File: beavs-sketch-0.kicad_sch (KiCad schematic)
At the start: 31 parts, among them J1 USB_C_Receptacle_USB2.0_16P, J3 Conn_01x02, J5 Conn_01x02, Q1 SiS402DN, Q2 SiS402DN, U15 SN74LVC8T245, U16 SRV05-4, U17 SRV05-4, U19 LM74502, U7 AMS1117-3.3, U8 AMS1117-5.0

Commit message: I may be stupid
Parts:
- removed C46: 220n, Capacitor_SMD:C_0402_1005Metric, symbol Device:C_Small
- removed R2: 100, Resistor_SMD:R_0402_1005Metric, symbol Device:R_Small
- removed U19: LM74502, Package_TO_SOT_SMD:SOT-23-8, symbol beavs-symbols:LM74502
- added Q3: AO3401A, Package_TO_SOT_SMD:SOT-23, symbol Transistor_FET:AO3401A
- added R14: R_Small, Resistor_SMD:R_0402_1005Metric, symbol Device:R_Small
- added R2: R, Resistor_SMD:R_0805_2012Metric, symbol Device:R
- added U19: LM74700, Package_TO_SOT_SMD:SOT-23-6, symbol Power_Management:LM74700
- C45: value 220n -> C_Small; LCSC C16772 -> (none)
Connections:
- net +BATT: now also U19.4 (CATHODE)
- net GND: now also U19.2 (GND)
- net at J3.2 (Pin_2), Q1.5 (D): now also R2.1
- net at Q1.4 (G): now also Q3.3 (D), R14.2; no longer Q2.4 (G)
- net at C45.1: now also Q1.1 (S), Q1.2 (S), Q1.3 (S), Q2.1 (S), Q2.2 (S), Q2.3 (S), R14.1, R2.2, U19.6 (ANODE)
- net at C45.2: now also U19.1 (VCAP)
- new net: Q2.4 (G), Q3.2 (S), U19.5 (GATE)
- new net mcu/SERVO_POWER_EN: Q3.1 (G)
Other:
- sheet mcu ports: added SERVO_POWER_EN; removed none
- moved on the sheet: C15, C16, C17, C18, D1, D2, D3, D4, D5, D6, D7, D8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

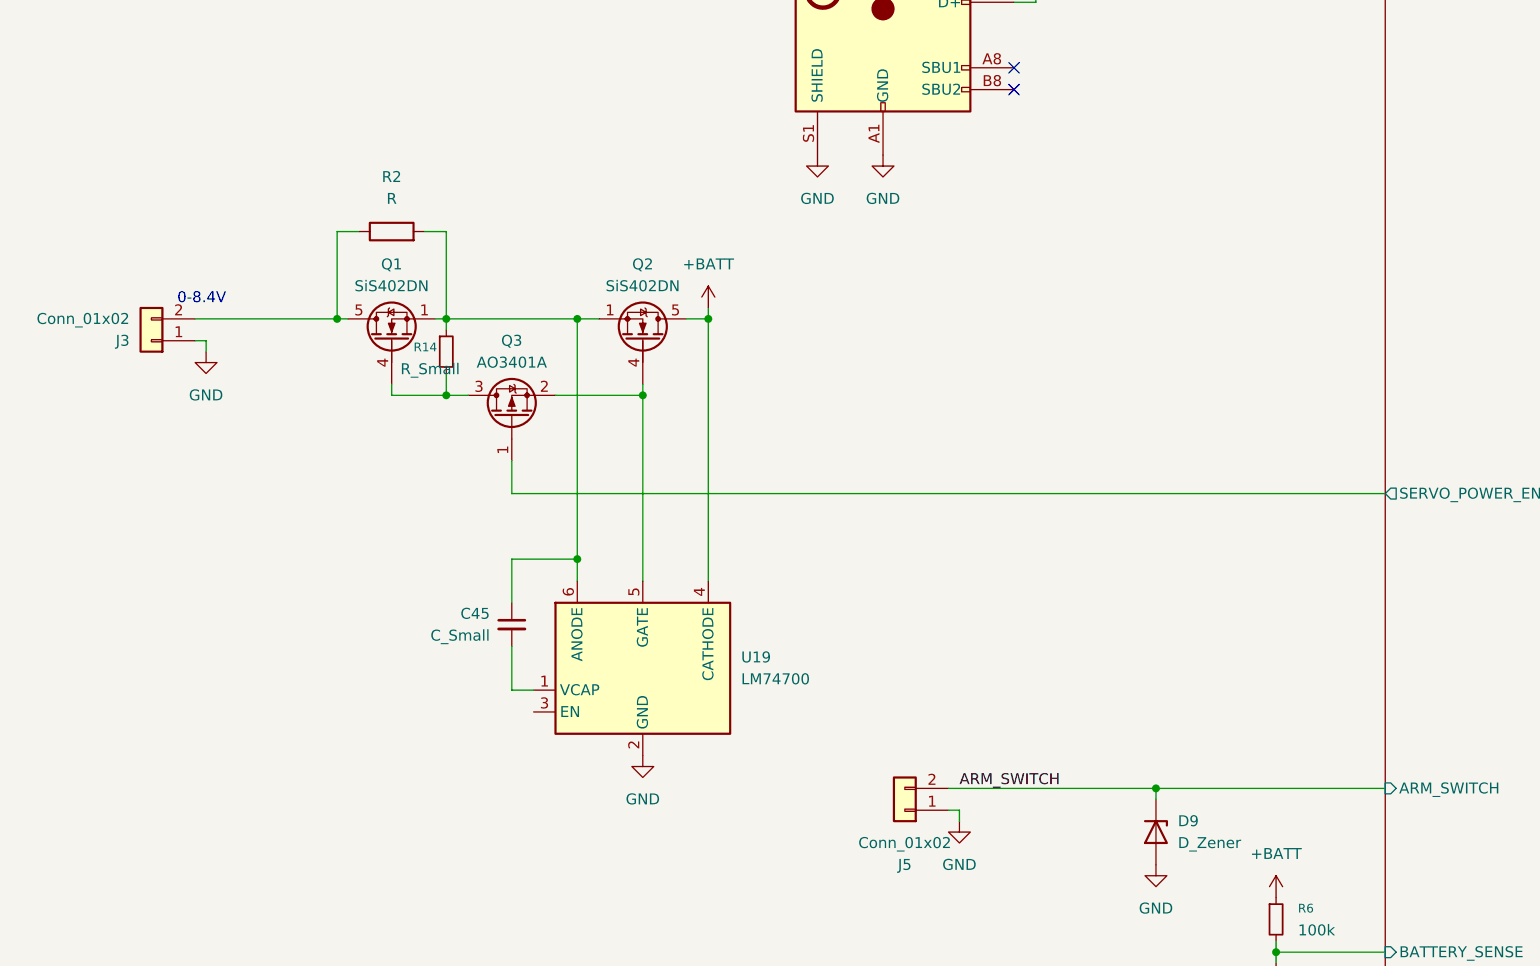
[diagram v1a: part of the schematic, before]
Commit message: definitely stupid
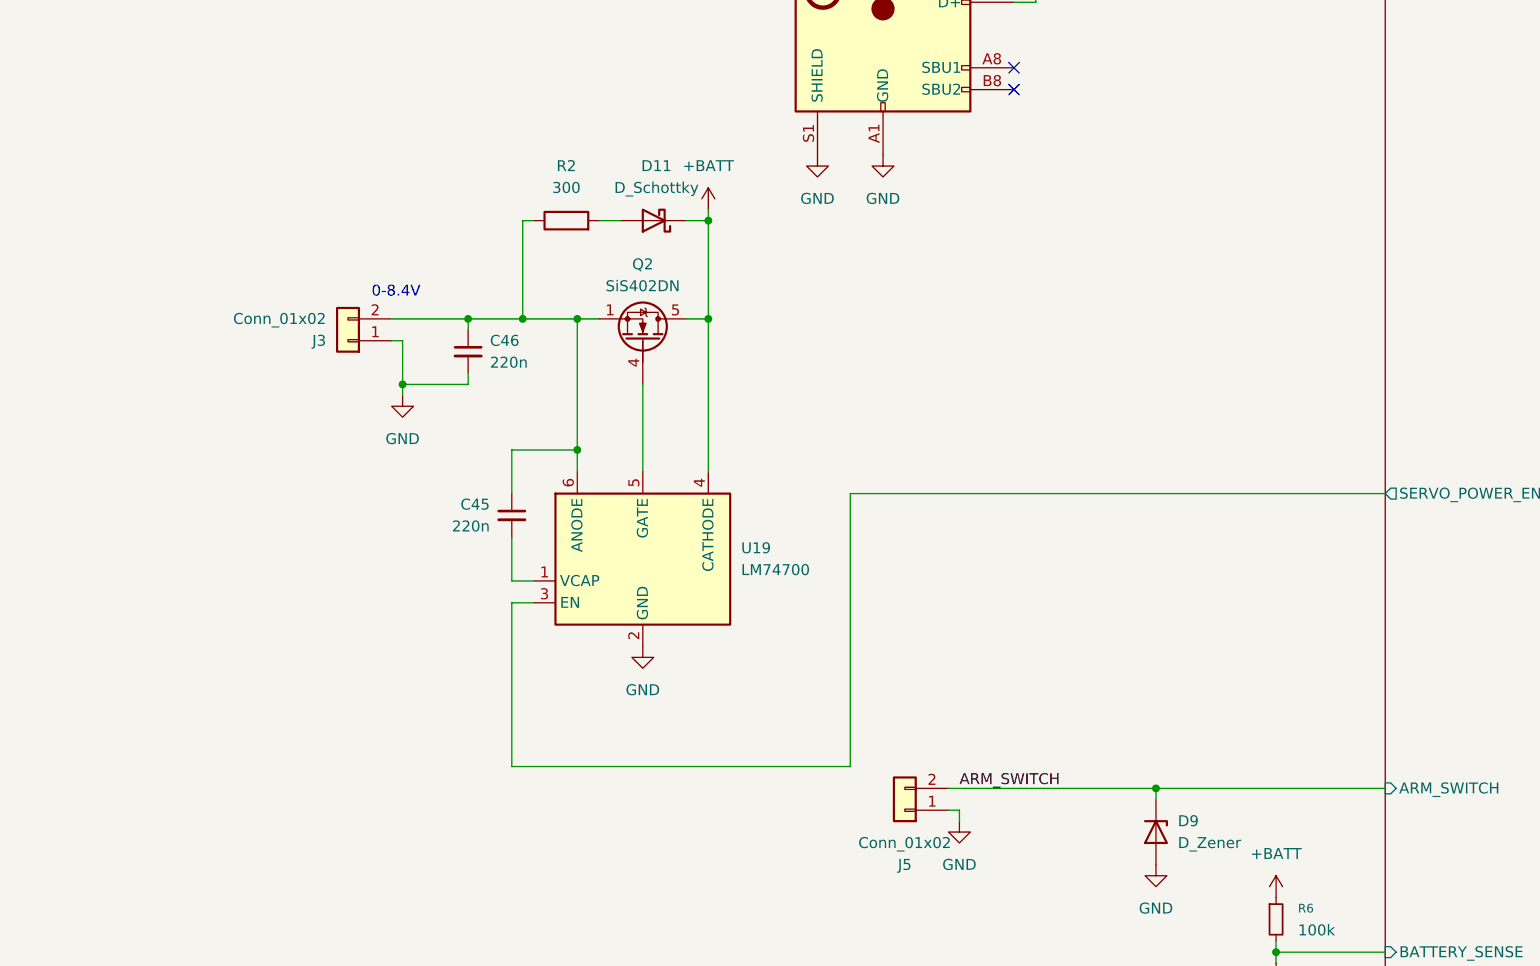
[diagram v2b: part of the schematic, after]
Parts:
- removed Q1: SiS402DN, Package_SO:Vishay_PowerPAK_1212-8_Single, symbol Transistor_FET:Q_NMOS_SSSGD_AvalancheRated
- removed Q3: AO3401A, Package_TO_SOT_SMD:SOT-23, symbol Transistor_FET:AO3401A
- removed R14: R_Small, Resistor_SMD:R_0402_1005Metric, symbol Device:R_Small
- added C46: 220n, Capacitor_SMD:C_0402_1005Metric, symbol Device:C_Small
- added D11: D_Schottky, Diode_SMD:D_SOD-123, symbol Device:D_Schottky
- C45: value C_Small -> 220n; LCSC (none) -> C16772
- R2: value R -> 300; footprint Resistor_SMD:R_0805_2012Metric -> Resistor_SMD:R_1206_3216Metric
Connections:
- net +BATT: now also D11.1 (K)
- net GND: now also C46.2
- net mcu/SERVO_POWER_EN: now also U19.3 (EN)
- net at C45.1, Q2.1 (S), Q2.2 (S)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: now also J3.2 (Pin_2), R2.1, C46.1; no longer R2.2
- new net: D11.2 (A), R2.2
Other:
- moved on the sheet: J3, R2, U19
